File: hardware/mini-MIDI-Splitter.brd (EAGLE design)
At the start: 140.8 x 19.1 mm, 40 parts, among them IC1 6N138, IC2 4050D, IC3 REG1117, X1 DIN5PIN, X2 DIN5PIN, X3 DIN5PIN, X4 DIN5PIN, X5 DIN5PIN, X6 DIN5PIN

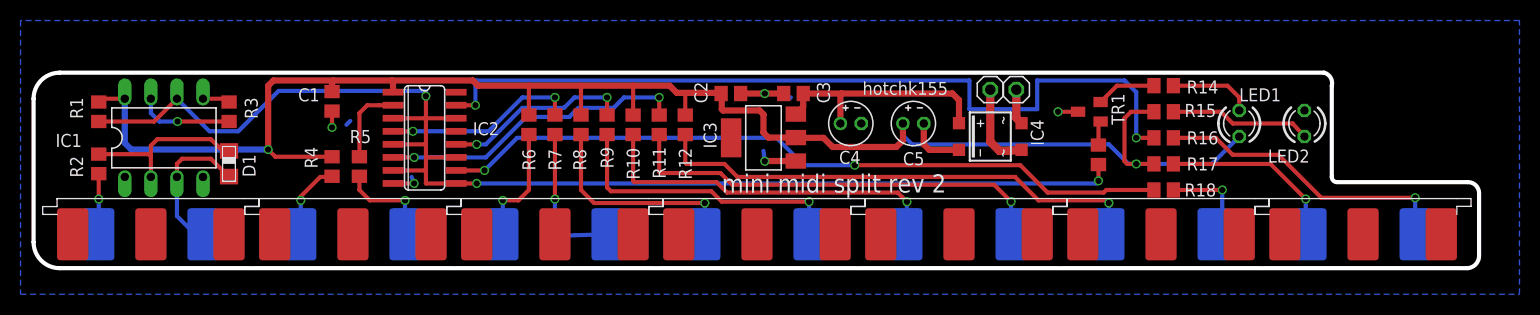
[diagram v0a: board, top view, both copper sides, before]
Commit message: REV3 PCB
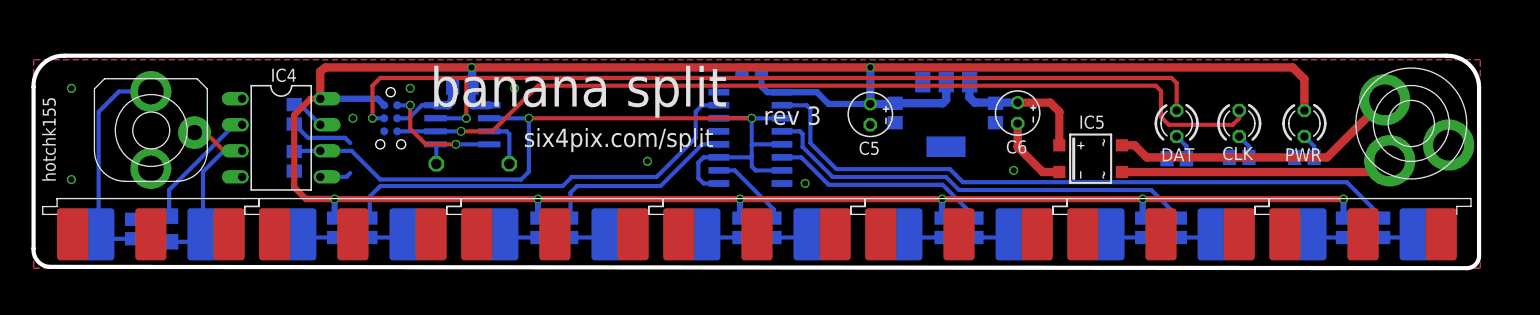
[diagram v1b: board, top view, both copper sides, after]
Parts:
- removed GND, VIN: (no value), pinhead:1X01
- removed TR1: (no value), transistor:SOT23-BEC
- added C6: 4u7, rcl:E2-4
- added DAT: (no value), led:LED3MM
- added IC5: (no value), microbuilder:SOIC-4
- added ICSP: (no value), tag-connect:TC2030-MCP-NL
- added RA2, RA4: (no value), pinhead:1X01
- added U$1: PWR_SOCKET_2_1MM, jason_eagle6:PWR_SOCKET_2_1MM
- added X7: VERTICAL_3_5MM_SOCKET, jason_eagle6:VERTICAL_3_5MM_SOCKET
- C1: value (none) -> 100n
- C3: value 100n -> (none)
- C4: value 4u7 -> 100n; device rcl:E2-4 -> rcl:C0805
- IC1: value 6N138 -> REG1117; device optocoupler:DIL08 -> burr-brown:SOT223
- IC3: value REG1117 -> PIC12F1822SO08; device burr-brown:SOT223 -> jasons_stuff:SO08
- IC4: value (none) -> 6N138; device microbuilder:SOIC-4 -> optocoupler:DIL08
- R1: value 1k8 -> 1k
- R13, R15: value 1k -> 220r
- R17, R18: value 220r -> 1k8
- R3: value 1k8 -> 220r
- moved R1 117.6 mm to (123.8, 10.8), flipped to the bottom, turned to 180 degrees
- moved R2 111.1 mm to (117.5, 10.8), flipped to the bottom, turned to 180 degrees
- moved R4 102.5 mm to (131.4, 3.94), flipped to the bottom, turned to 270 degrees
- moved R16 100.8 mm to (9.65, 3.81), flipped to the bottom, turned to 90 degrees
- moved R5 96.1 mm to (127.6, 3.94), flipped to the bottom, turned to 90 degrees
- moved R3 92.4 mm to (111.4, 10.7), flipped to the bottom, turned to 180 degrees
- moved R17 84.8 mm to (25.4, 15.0), flipped to the bottom, turned to 90 degrees
- moved R18 84.8 mm to (25.4, 10.4), flipped to the bottom, turned to 90 degrees
- moved R15 81.6 mm to (29.3, 3.94), flipped to the bottom, turned to 90 degrees
- moved R14 78.6 mm to (32.8, 3.94), flipped to the bottom, turned to 270 degrees
- moved IC1 76.2 mm to (88.9, 15.0), flipped to the bottom, turned to 180 degrees
- moved IC4 69.1 mm to (24.1, 12.7), turned to 270 degrees
- moved C1 64.7 mm to (93.7, 15.1), flipped to the bottom
- moved R6 64.2 mm to (111.6, 3.94), flipped to the bottom, turned to 270 degrees
- moved R7 58.1 mm to (108.1, 3.94), flipped to the bottom, turned to 90 degrees
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- renumbered LED1 to CLK, LED2 to PWR
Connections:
- removed net DAT: IC1.6, IC2.11, IC2.14, IC2.3, IC2.5, IC2.7, IC2.9, R1.2, R13.2
- removed net N$26: PWR.A, R15.1
- new net CLK: CLK.K, R2.2
- new net CLK_LED: CLK.A, IC3.6, ICSP.5
- new net DAT_LED: DAT.A, IC3.7, ICSP.4
- new net MIDI_IN: IC2.11, IC2.14, IC2.3, IC2.5, IC2.7, IC2.9, IC3.2, IC4.6, R18.2
- new net MIDI_OUT: IC3.3, RA4.1
- new net N$33: IC3.4, ICSP.1
- net GND: now also C4.2, C6.-, IC1.1, IC3.8, IC4.5, IC5.-, ICSP.3, R1.1, R17.1, R2.1; no longer C4.-, IC1.5, IC3.1, IC4.-, PWR.K, TR1.C
- net N$1: now also R14.2; no longer R5.2
- net N$10: now also R8.1; no longer R11.1
- net N$11: now also IC2.2, R4.1; no longer IC2.4, R7.1
- net N$12: now also IC2.4, R6.1; no longer IC2.2, R5.1
- net N$13: now also PWR.K, R1.2; no longer R14.1, TR1.E
- net N$14: now also R15.1; no longer R4.1
- net N$15: now also R13.1; no longer R6.1
- net N$16: now also R11.1; no longer R8.1
- net N$17: now also R9.1; no longer R10.1
- net N$18: now also R7.1; no longer R12.1
- net N$19: now also R5.1; no longer R17.1
- net N$2: now also R12.2; no longer R7.2
- net N$20: now also R16.1, X7.4; no longer R2.1
- net N$21: now also IC4.2, R16.2; no longer IC1.2, R2.2
- net N$22: now also IC4.7, R17.2; no longer IC1.7, R3.2
- net N$23: now also DAT.K, R3.2; no longer CLK.K, R14.2
- net N$24: now also IC4.3, X7.3; no longer IC1.3
- net N$25: now also IC3.5, RA2.1; no longer R13.1, TR1.B
- net N$27: now also IC5.~1, U$1.BARREL; no longer IC4.~1, VIN.1
- net N$28: now also IC5.~2, U$1.PIN; no longer GND.1, IC4.~2
- net N$3: now also R10.2; no longer R9.2
- net N$4: now also R8.2; no longer R11.2
- net N$5: now also R6.2; no longer R18.2
- net N$6: now also R4.2; no longer R16.2
- net N$7: now also R14.1; no longer R16.1
- net N$8: now also R12.1; no longer R9.1
- net N$9: now also R10.1; no longer R18.1
- net VCC: now also C3.1, C4.1, IC1.2, IC3.1, IC4.8, ICSP.2, PWR.A, R11.2, R13.2, R18.1, R5.2, R7.2, R9.2; no longer C1.1, CLK.A, IC1.8, IC3.2, R1.1, R10.2, R12.2, R17.2, R4.2, R6.2, R8.2
- net VIN: now also C1.1, C6.+, IC1.3, IC5.+; no longer C3.1, C4.+, IC3.3, IC4.+
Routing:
- net DAT: track 127.5 -> 0.00 mm, vias 3 -> 0
- net VCC: track 162.4 -> 269.7 mm, vias 2 -> 8
- net DAT_LED: track 0.00 -> 92.9 mm, vias 0 -> 2
- net CLK_LED: track 0.00 -> 88.0 mm, vias 0 -> 1
- net MIDI_IN: track 0.00 -> 81.3 mm, vias 0 -> 2
- net N$9: track 71.6 -> 7.77 mm, vias 2 -> 0
- net N$11: track 18.9 -> 65.0 mm, vias 2 -> 0
- net N$18: track 48.7 -> 3.43 mm, vias 1 -> 0
- net N$7: track 80.9 -> 41.3 mm, vias 2 -> 0
- net N$4: track 43.1 -> 3.56 mm, vias 1 -> 0
- net N$12: track 7.85 -> 43.0 mm
- net N$17: track 35.2 -> 3.56 mm, vias 1 -> 0
- net N$6: track 29.5 -> 3.31 mm, vias 1 -> 0
- net N$3: track 28.6 -> 3.56 mm, vias 1 -> 0
- net N$28: track 3.48 -> 28.4 mm
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- added copper zone on layer 1, net GND
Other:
- board size 140.8 x 19.1 mm -> 140.8 x 20.7 mm
- board text added: "banana split"
- board text added: "rev 3"
- board text added: "six4pix.com/split"
- board text removed: "mini midi split rev 2"
